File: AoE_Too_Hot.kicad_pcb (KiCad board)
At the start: 2 copper layers, 8 parts, among them U1 LMV393

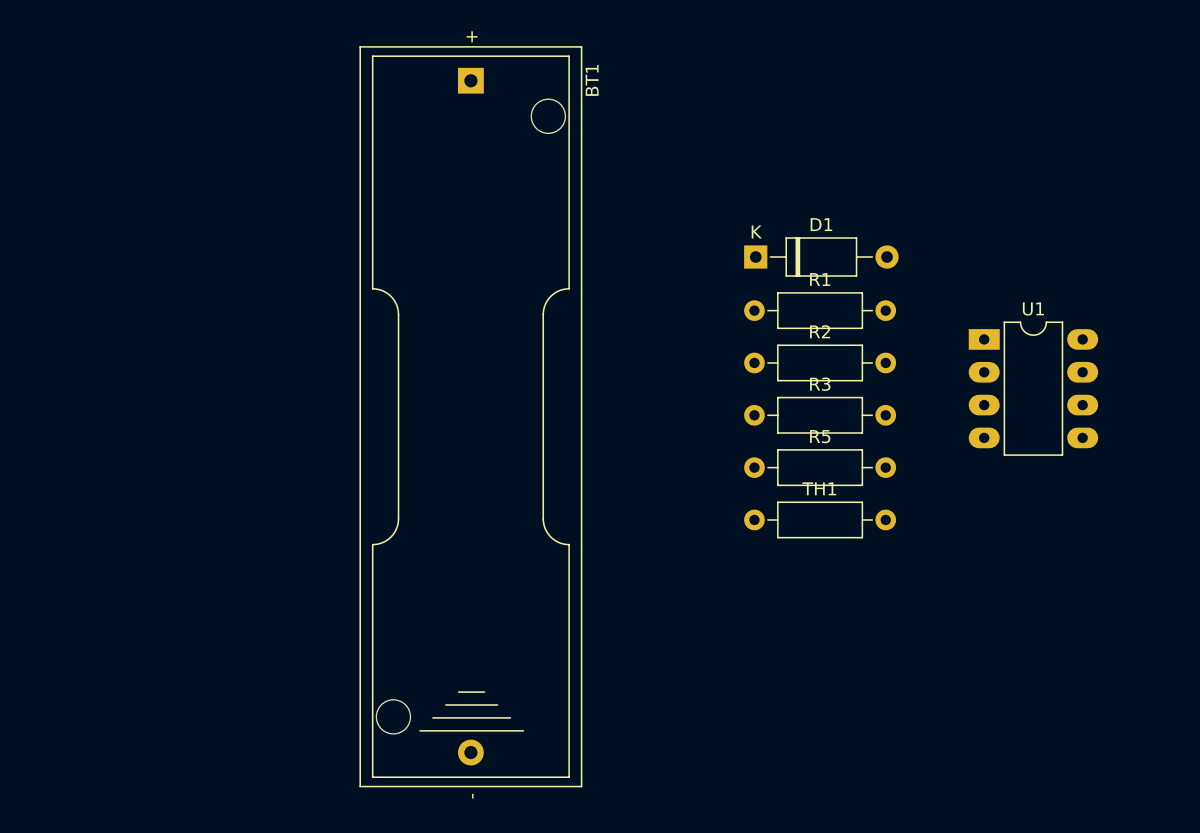
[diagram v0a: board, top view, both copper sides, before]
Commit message: Add files via upload
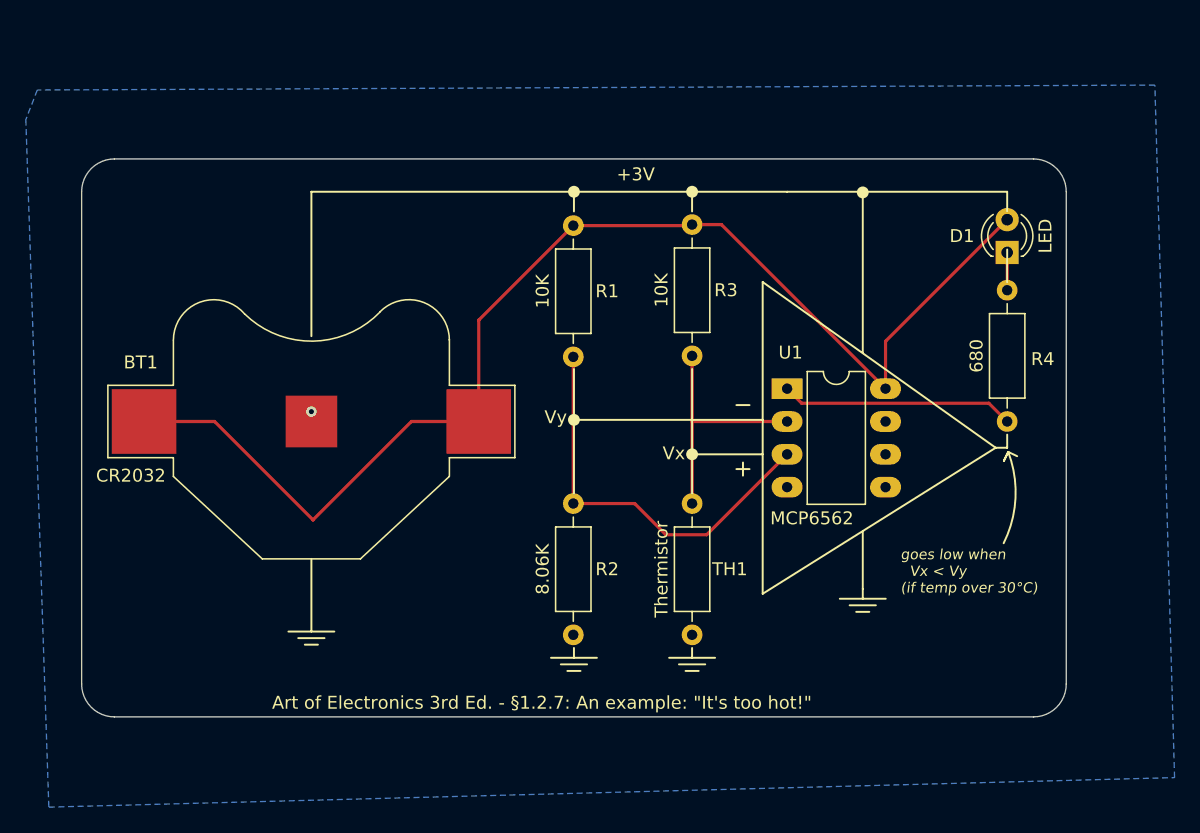
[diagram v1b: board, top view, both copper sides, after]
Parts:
- BT1: footprint Battery:BatteryHolder_Keystone_2460_1xAA -> Battery:BatteryHolder_Multicomp_BC-2001_1x2032
- D1: footprint Diode_THT:D_A-405_P10.16mm_Horizontal -> LED_THT:LED_D3.0mm_IRBlack
- U1: value LMV393 -> MCP6562
- moved BT1 29.1 mm to (94.0, 78.7), turned to 0 degrees
- moved R4 23.9 mm to (147.8, 68.6), turned to -90 degrees
- moved D1 19.5 mm to (147.8, 65.7), turned to 90 degrees
- moved R2 17.7 mm to (114.2, 85.1), turned to -90 degrees
- moved U1 15.7 mm to (130.8, 76.2)
- moved R3 15.5 mm to (123.4, 63.5), turned to -90 degrees
- moved R1 15.5 mm to (114.2, 63.6), turned to -90 degrees
- moved TH1 4.99 mm to (123.4, 85.1), turned to -90 degrees
- renumbered R5 to R4
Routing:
- net Net-(BT1-+): track 0.00 -> 96.8 mm
- net Net-(U1A-+): track 0.00 -> 31.5 mm
- net Net-(U1A--): track 0.00 -> 18.8 mm
- net Net-(R4-Pad2): track 0.00 -> 18.1 mm
- net Net-(D1-K): track 0.00 -> 2.92 mm
- net GND: track 0.00 -> 0.76 mm, vias 0 -> 1
- added copper zone on B.Cu, net GND
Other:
- board outline added: 76.2 x 43.2 mm
- board text added: "+3V"
- board text added: "Art of Electronics 3rd Ed. - §1.2.7: An example: {dblquote}It's too hot!{dblquote}"
- board text added: "Shamelessly copied from the 3rd Ed of AoE. Voltage divider R1/R2 gives Vy, constant voltage. Voltage divider R3/TH1 gives Vx, voltage that changes with temperature. The NTC thermistor decreases in resistance as temperature increases. The comparator's output goes low when Vx is greater than Vy. Thermistor - 103JG1F"
- board text added: "Vx"
- board text added: "Vy"
- board text added: "github.com/b0xmaker/AoE_TooHot Designed in NC. 2024-01-09"
- board text added: "goes low when Vx < Vy (if temp over 30°C)"
